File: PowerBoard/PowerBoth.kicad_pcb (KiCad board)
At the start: 2 copper layers, 141.8 x 24.9 mm, 54 parts, among them J101 2X10-2MMSMD, J201 PJ-079AH, J202 2MM-1X5, M201 IRF7205, Q101 IRF7205, U201 LTC4002ES8-4.2PBFSO-8_S-M, U301 MP2307DN-LF, U401 TPS61030RSAR

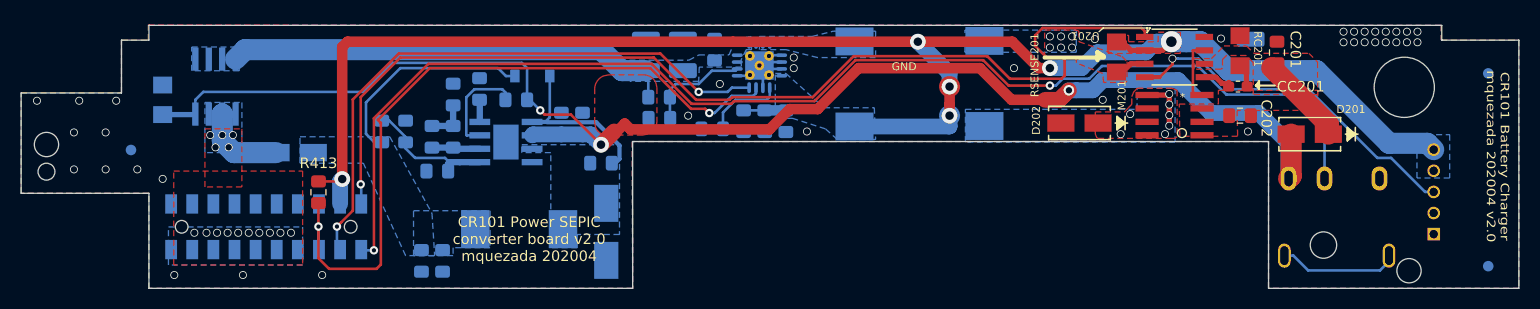
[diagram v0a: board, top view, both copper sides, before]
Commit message: Buck/boost v4.0.
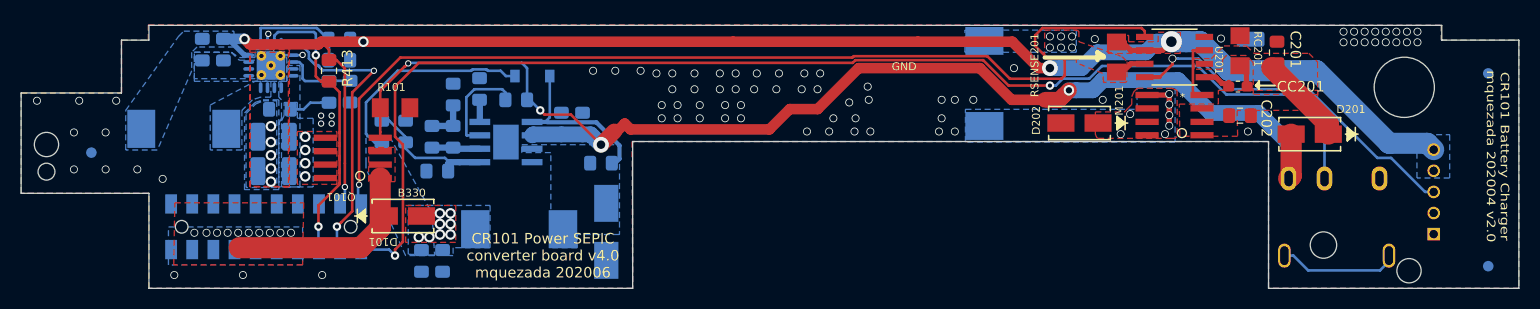
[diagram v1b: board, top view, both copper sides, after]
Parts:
- C2A301, C2B301: value 10uF -> 22uF
- C301: value 0.1uF -> 10nF
- C3A301: value 3.9uF -> 3.9nF
- C3B301: value 0.01uF -> (0.01uF)
- D101, Q101, R101: moved to F.Cu
- D301: value B130 -> (B130)
- Dbs301: value 1N4148 -> (1N4148)
- moved L401 63.6 mm to (149.5, 130.8), turned to 180 degrees
- moved C401 53.7 mm to (151.2, 123.2)
- moved C404 53.7 mm to (153.2, 123.2)
- moved U401 46.2 mm to (157.8, 124.8), turned to 90 degrees
- moved C402 41.5 mm to (158.6, 128.9), turned to 180 degrees
- moved C406 40.3 mm to (158.0, 134.8), turned to 180 degrees
- moved R401 39.1 mm to (164.2, 122.2), turned to 0 degrees
- moved C403 36.1 mm to (158.0, 131.5), turned to 180 degrees
- moved R402 35.9 mm to (164.2, 124.2), turned to 180 degrees
- moved R403 31.3 mm to (163.2, 127.2), turned to 270 degrees
- moved R404 29.4 mm to (165.2, 127.2), turned to 90 degrees
- moved R101 22.0 mm to (169.5, 128.8), turned to 180 degrees
- moved Q101 14.6 mm to (165.5, 133.5), turned to 90 degrees
- moved D101 11.9 mm to (170.2, 139.0)
- moved R413 11.5 mm to (163.2, 125.2), turned to 90 degrees
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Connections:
- net Net-(L401-Pad1) renamed /PowerBoost1000/SW
- net Net-(R401-Pad1) renamed /PowerBoost1000/LBI
- net Net-(R403-Pad1) renamed /PowerBoost1000/FB
- R413 pad 1: /VBATT -> /EN_PB
- R413 pad 2: /EN_PB -> /VBATT
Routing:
- net /EN_PB: track 68.6 -> 27.5 mm
- net /FromBoost: track 42.6 -> 3.88 mm, vias 0 -> 4
- net /LBO: track 56.3 -> 28.7 mm
- net /V+CH: track 137.1 -> 119.2 mm, vias 3 -> 4
- net 5V: track 8.10 -> 18.9 mm, vias 15 -> 10
- net GND: track 13.7 -> 4.51 mm, vias 38 -> 89
- net /VBATT: track 155.4 -> 148.6 mm, vias 6 -> 5
- net /CHSTAT: track 100.0 -> 96.9 mm
- net /PowerBoost1000/FB: track 9.94 -> 7.64 mm
- net /PowerBoost1000/LBI: track 9.54 -> 10.3 mm
- net /FromBuck: track 20.6 -> 20.5 mm, vias 0 -> 8
- added copper zone on F.Cu, net /FromBoost
- added copper zone on F.Cu, net /FromBuck
- added copper zone on B.Cu, net GNDPWR
- added copper zone on F.Cu, net GNDPWR
- removed copper zone on F.Cu, net /V+CH
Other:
- board text added: "CR101 Power SEPIC converter board v4.0 mquezada 202006"
- board text removed: "CR101 Power SEPIC converter board v2.0 mquezada 202004"
